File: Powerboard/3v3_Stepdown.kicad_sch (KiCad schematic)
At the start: 16 parts, among them U1 MP2338GTL-Z

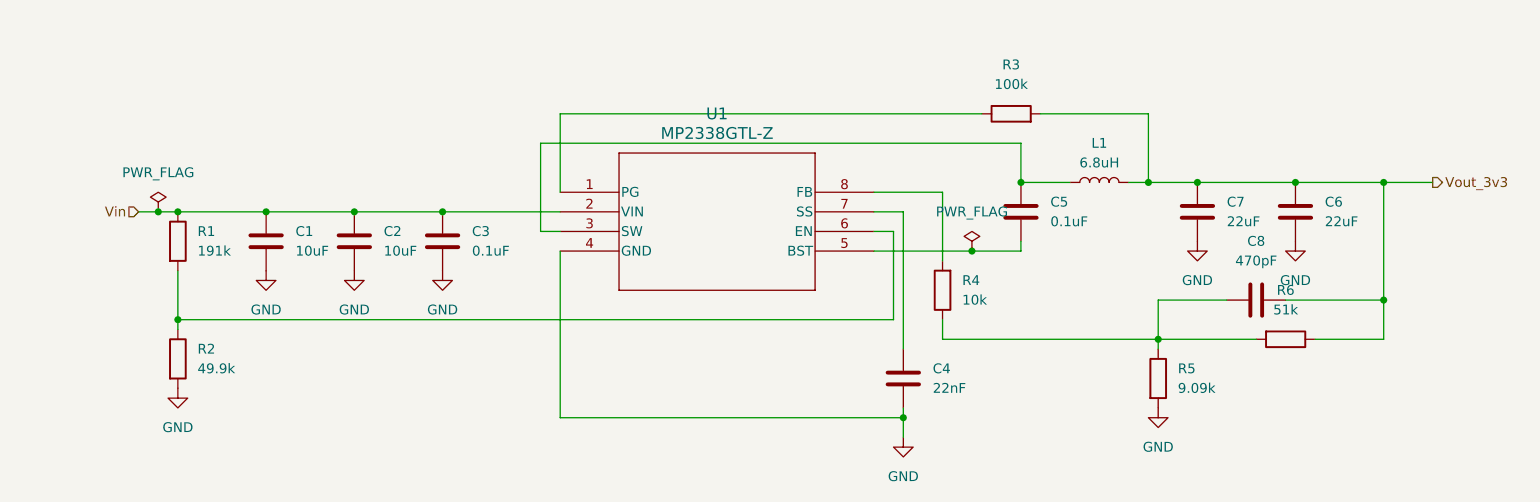
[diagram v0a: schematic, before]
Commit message: Updated
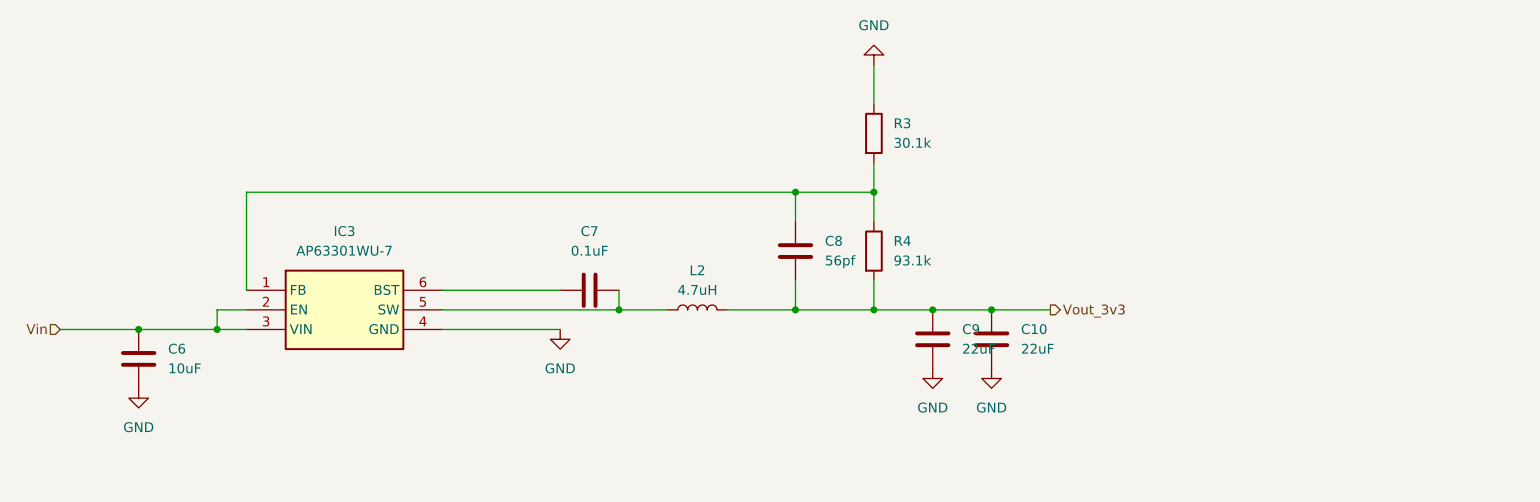
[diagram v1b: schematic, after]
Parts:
- removed C1, C2: 10uF, Capacitor_SMD:C_1206_3216Metric, symbol Device:C
- removed C3, C5: 0.1uF, Capacitor_SMD:C_0603_1608Metric, symbol Device:C
- removed C4: 22nF, Capacitor_SMD:C_0603_1608Metric, symbol Device:C
- removed L1: 6.8uH, Inductor_SMD:L_Bourns_SRP7028A_7.3x6.6mm, symbol Device:L
- removed R1: 191k, Resistor_SMD:R_0603_1608Metric, symbol Device:R
- removed R2: 49.9k, Resistor_SMD:R_0603_1608Metric, symbol Device:R
- removed R5: 9.09k, Resistor_SMD:R_0603_1608Metric, symbol Device:R
- removed R6: 51k, Resistor_SMD:R_0603_1608Metric, symbol Device:R
- removed U1: MP2338GTL-Z, MP2338GTL:SOT583_MP2338_MNP, symbol MP2338GTL:MP2338GTL-Z
- added C10, C9: 22uF, Capacitor_SMD:C_1206_3216Metric, symbol Device:C
- added IC3: AP63301WU-7, AP63301WU:SOT95P280X100-6N, symbol AP63301WU:AP63301WU-7
- added L2: 4.7uH, Inductor_SMD:L_Bourns_SRP7028A_7.3x6.6mm, symbol Device:L
- C6: value 22uF -> 10uF; footprint Capacitor_SMD:C_1206_3216Metric -> Capacitor_SMD:C_1210_3225Metric
- C7: value 22uF -> 0.1uF; footprint Capacitor_SMD:C_1206_3216Metric -> Capacitor_SMD:C_0603_1608Metric
- C8: value 470pF -> 56pf; footprint Capacitor_SMD:C_0603_1608Metric -> Capacitor_SMD:C_0201_0603Metric
- R3: value 100k -> 30.1k
- R4: value 10k -> 93.1k
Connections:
- net GND: now also R3.1, C10.2, C9.2, IC3.4 (GND); no longer C7.2
- net Vin: now also C6.1, IC3.2 (EN), IC3.3 (VIN)
- net Vout_3v3: now also R4.2, C10.1, C9.1, L2.2; no longer C6.1, C7.1, R3.2
- net at C8.1, R4.1: now also R3.2, IC3.1 (FB)
- new net: C7.2, IC3.5 (SW), L2.1
- new net: C7.1, IC3.6 (BST)
